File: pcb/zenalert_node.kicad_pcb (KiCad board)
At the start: 2 copper layers, 65 x 55 mm, 9 parts, among them J1 MQ135, J2 MQ2, J3 DHT22, J4 OLED_SSD1306, U1 ESP32-S2-Mini

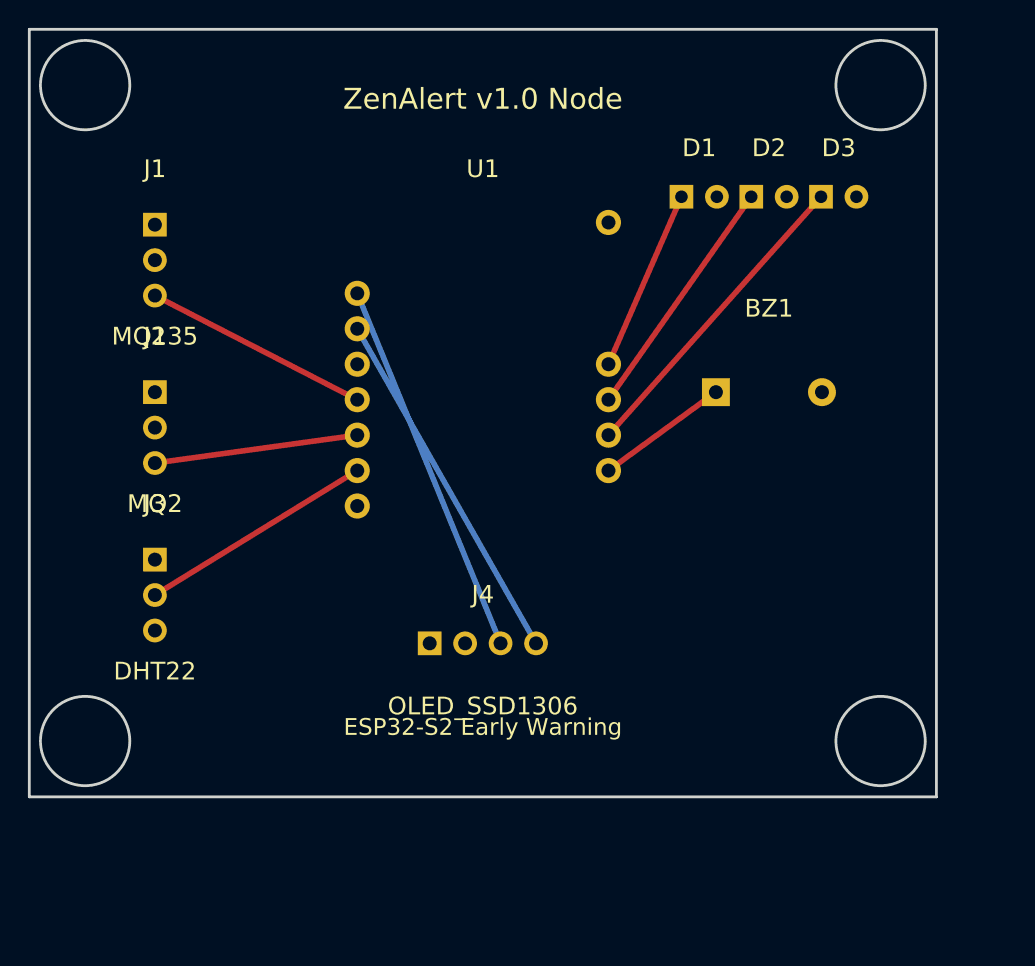
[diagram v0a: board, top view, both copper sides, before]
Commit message: feat (pcb) : add kicad design files production gerber and hardware documentation
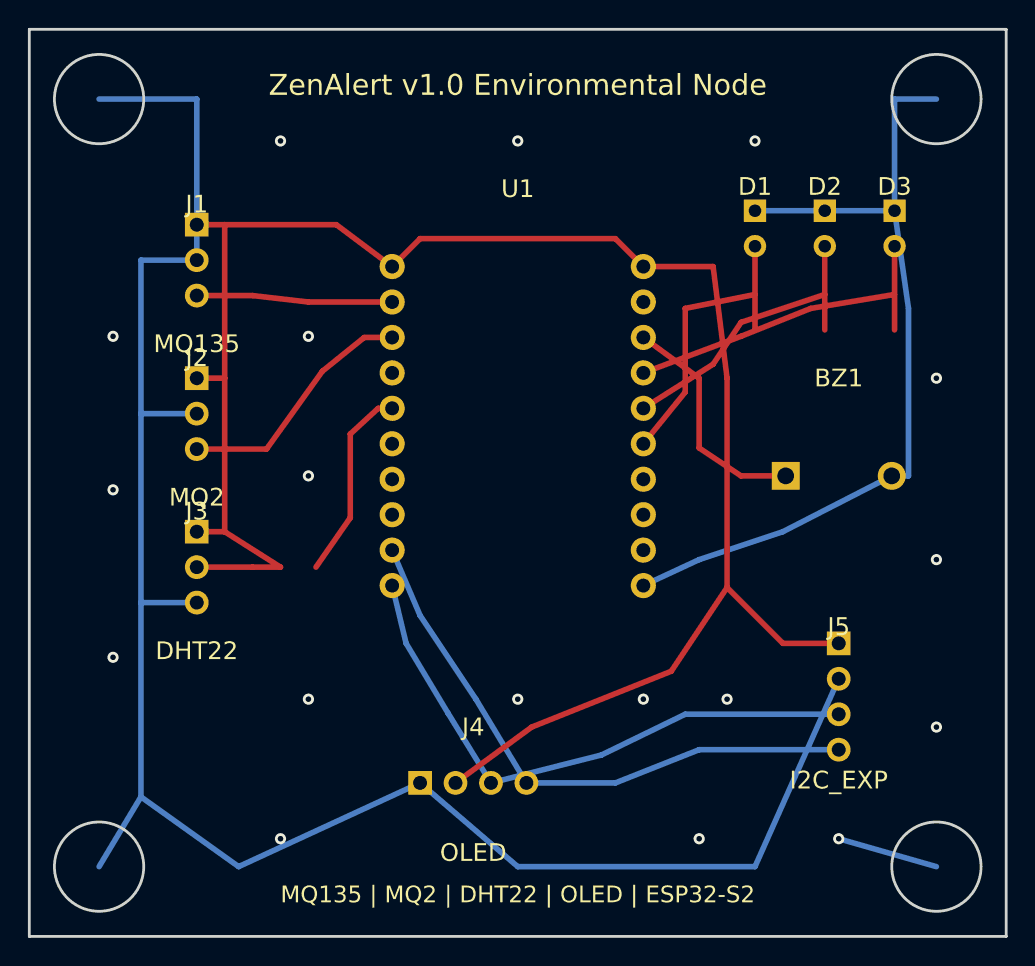
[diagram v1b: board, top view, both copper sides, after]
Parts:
- added J5: I2C_EXP, Connector_PinHeader:PinHeader_1x04_P2.54mm, F.Cu at (58.0, 47.8)
- J1, J2, J3: footprint Connector_PinHeader_2.54mm:PinHeader_1x03_P2.54mm_Vertical -> Connector_PinHeader:PinHeader_1x03_P2.54mm
- J4: value OLED_SSD1306 -> OLED; footprint Connector_PinHeader_2.54mm:PinHeader_1x04_P2.54mm_Vertical -> Display:SSD1306_OLED_0.96_I2C
- moved J4 10.0 mm to (31.8, 54.0)
- moved BZ1 7.81 mm to (58.0, 32.0)
- moved U1 5.09 mm to (35.0, 28.4)
- moved D1 4.60 mm to (52.0, 14.3)
- moved D2 4.60 mm to (57.0, 14.3)
- moved D3 4.60 mm to (62.0, 14.3)
- moved J1 3.93 mm to (12.0, 16.5)
- moved J2 3.37 mm to (12.0, 27.5)
- moved J3 3.05 mm to (12.0, 38.5)
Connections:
- net NET_MQ135_AOUT renamed MQ135_AOUT
- net NET_MQ2_AOUT renamed MQ2_AOUT
- BZ1 pad 1: NET_BUZZER -> BUZZER_ALARM
- D1 pad 1: NET_LED_GREEN -> LED_GREEN
- D2 pad 1: NET_LED_YELLOW -> LED_YELLOW
- D3 pad 1: NET_LED_RED -> LED_RED
- J3 pad 2: NET_DHT22_DATA -> DHT22_DATA
- J4 pad 3: NET_I2C_SCL -> I2C_SCL
- J4 pad 4: NET_I2C_SDA -> I2C_SDA
- U1 pad 10: NET_LED_RED -> I2C_SCL
- U1 pad 11: NET_BUZZER -> (no net)
- U1 pad 12: GND -> (no net)
- U1 pad 4: NET_DHT22_DATA -> (no net)
- U1 pad 5: (no net) -> DHT22_DATA
- U1 pad 6: NET_I2C_SDA -> (no net)
- U1 pad 7: NET_I2C_SCL -> (no net)
- U1 pad 8: NET_LED_GREEN -> (no net)
- U1 pad 9: NET_LED_YELLOW -> I2C_SDA
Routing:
- net (no net): track 0.00 -> 555.8 mm
- net NET_I2C_SCL: track 27.1 -> 0.00 mm
- net NET_I2C_SDA: track 25.9 -> 0.00 mm
- net NET_LED_RED: track 22.9 -> 0.00 mm
- net NET_LED_YELLOW: track 17.8 -> 0.00 mm
- net NET_DHT22_DATA: track 17.0 -> 0.00 mm
- net MQ135_AOUT: track 16.3 -> 0.00 mm
- net MQ2_AOUT: track 14.6 -> 0.00 mm
- net NET_LED_GREEN: track 13.1 -> 0.00 mm
- net NET_BUZZER: track 9.53 -> 0.00 mm
- net GND: vias 0 -> 18
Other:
- board size 65 x 55 mm -> 70 x 65 mm
- board text added: "MQ135 | MQ2 | DHT22 | OLED | ESP32-S2"
- board text added: "ZenAlert v1.0 Environmental Node"
- board text removed: "ESP32-S2 Early Warning"
- board text removed: "ZenAlert v1.0 Node"
